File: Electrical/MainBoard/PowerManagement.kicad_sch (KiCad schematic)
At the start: 71 parts, among them Q1 AO3401A, U5 TPS65131RGE, U6 TPS2121RUXR, U7 TPS7A9401DSCR, U8 LM61460AASQRJRRQ1

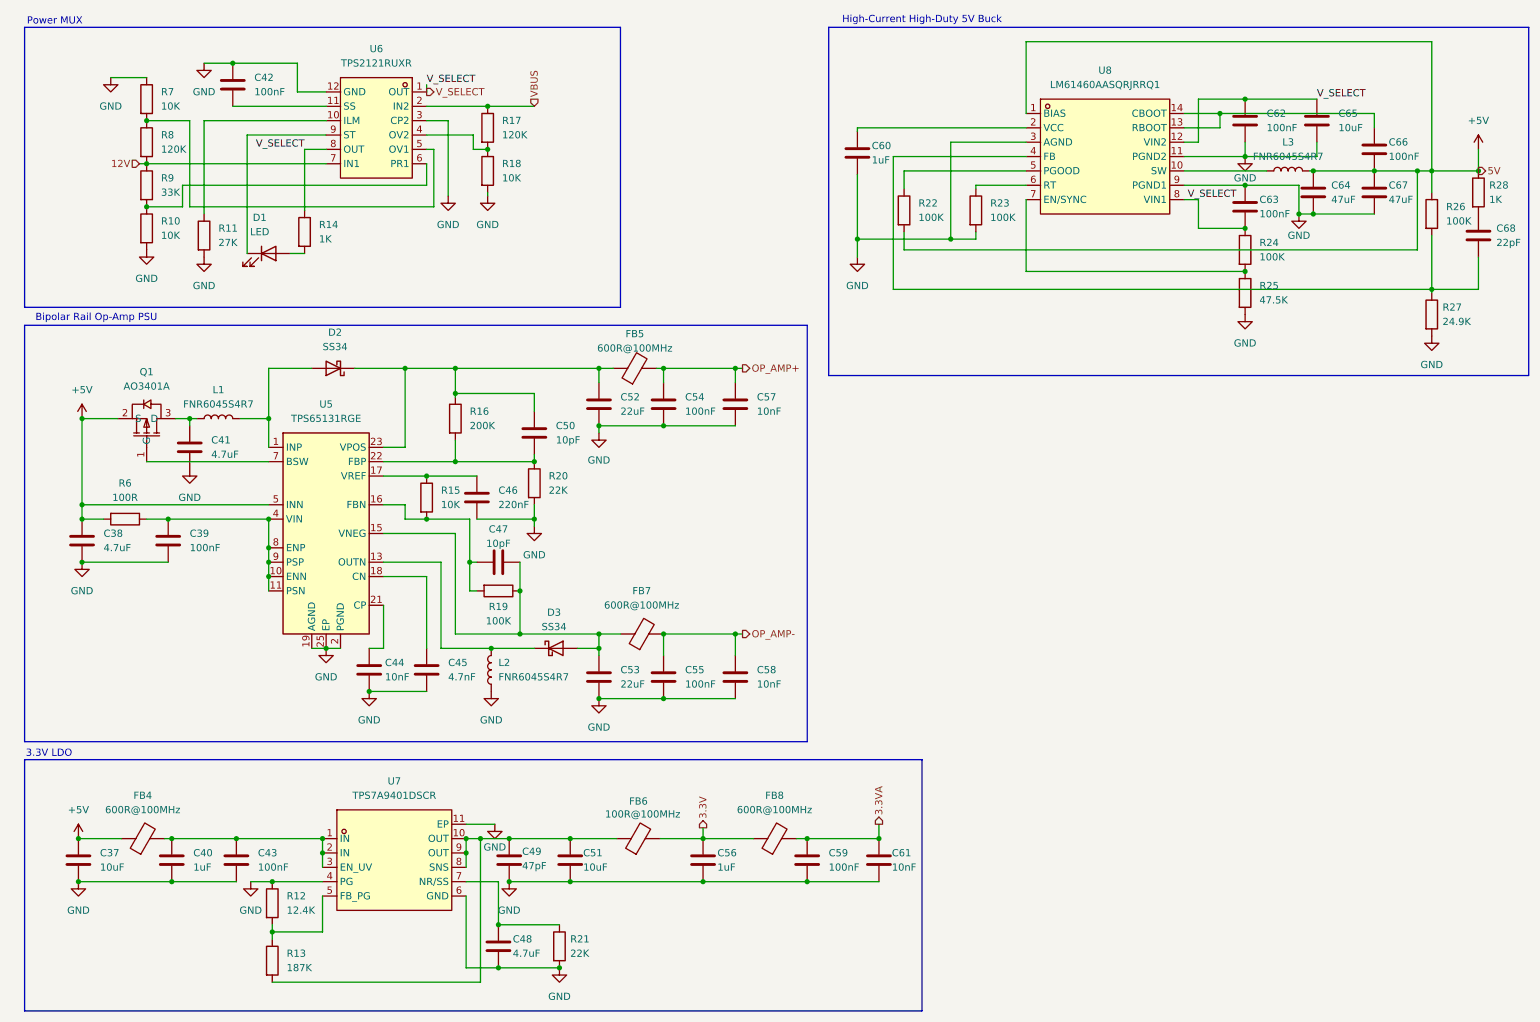
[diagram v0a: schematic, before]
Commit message: layout main
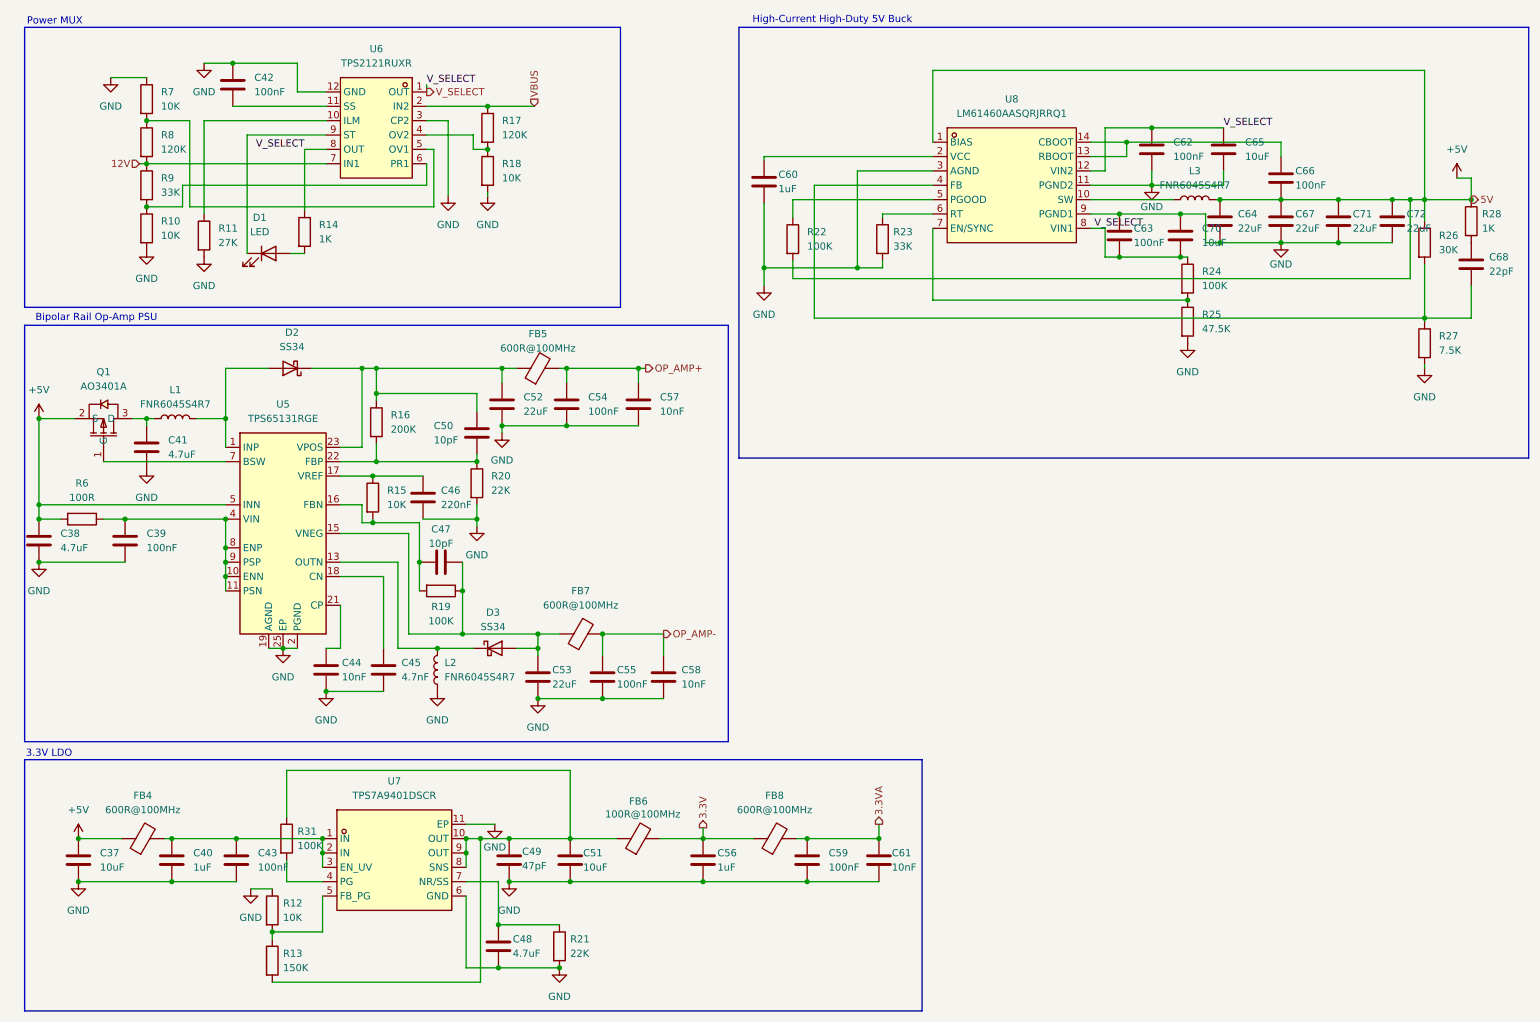
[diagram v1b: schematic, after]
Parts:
- added C70: 10uF, Capacitor_SMD:C_0603_1608Metric, symbol Device:C
- added C71, C72: 22uF, Capacitor_SMD:C_0805_2012Metric, symbol Device:C
- added R31: 100K, Resistor_SMD:R_0402_1005Metric, symbol Device:R
- C64, C67: value 47uF -> 22uF
- R10, R17, R18, R7, R8, R9: footprint Resistor_SMD:R_0402_1005Metric -> Resistor_SMD:R_0603_1608Metric
- R12: value 12.4K -> 10K; footprint Resistor_SMD:R_0603_1608Metric -> Resistor_SMD:R_0402_1005Metric
- R13: value 187K -> 150K
- R23: value 100K -> 33K
- R26: value 100K -> 30K; footprint Resistor_SMD:R_0402_1005Metric -> Resistor_SMD:R_0603_1608Metric
- R27: value 24.9K -> 7.5K
- R6: footprint Resistor_SMD:R_0603_1608Metric -> Resistor_SMD:R_0402_1005Metric
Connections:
- net +5V: now also C71.1, C72.1
- net GND: now also C70.1, C71.2, C72.2; no longer U7.4 (PG)
- net V_SELECT: now also C70.2
- net at C49.1, C51.1, FB6.1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: now also R31.1
- new net: R31.2, U7.4 (PG)
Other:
- moved on the sheet: C38, C39, C41, C44, C45, C46, C47, C50, C52, C53, C54, C55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

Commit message: new layout
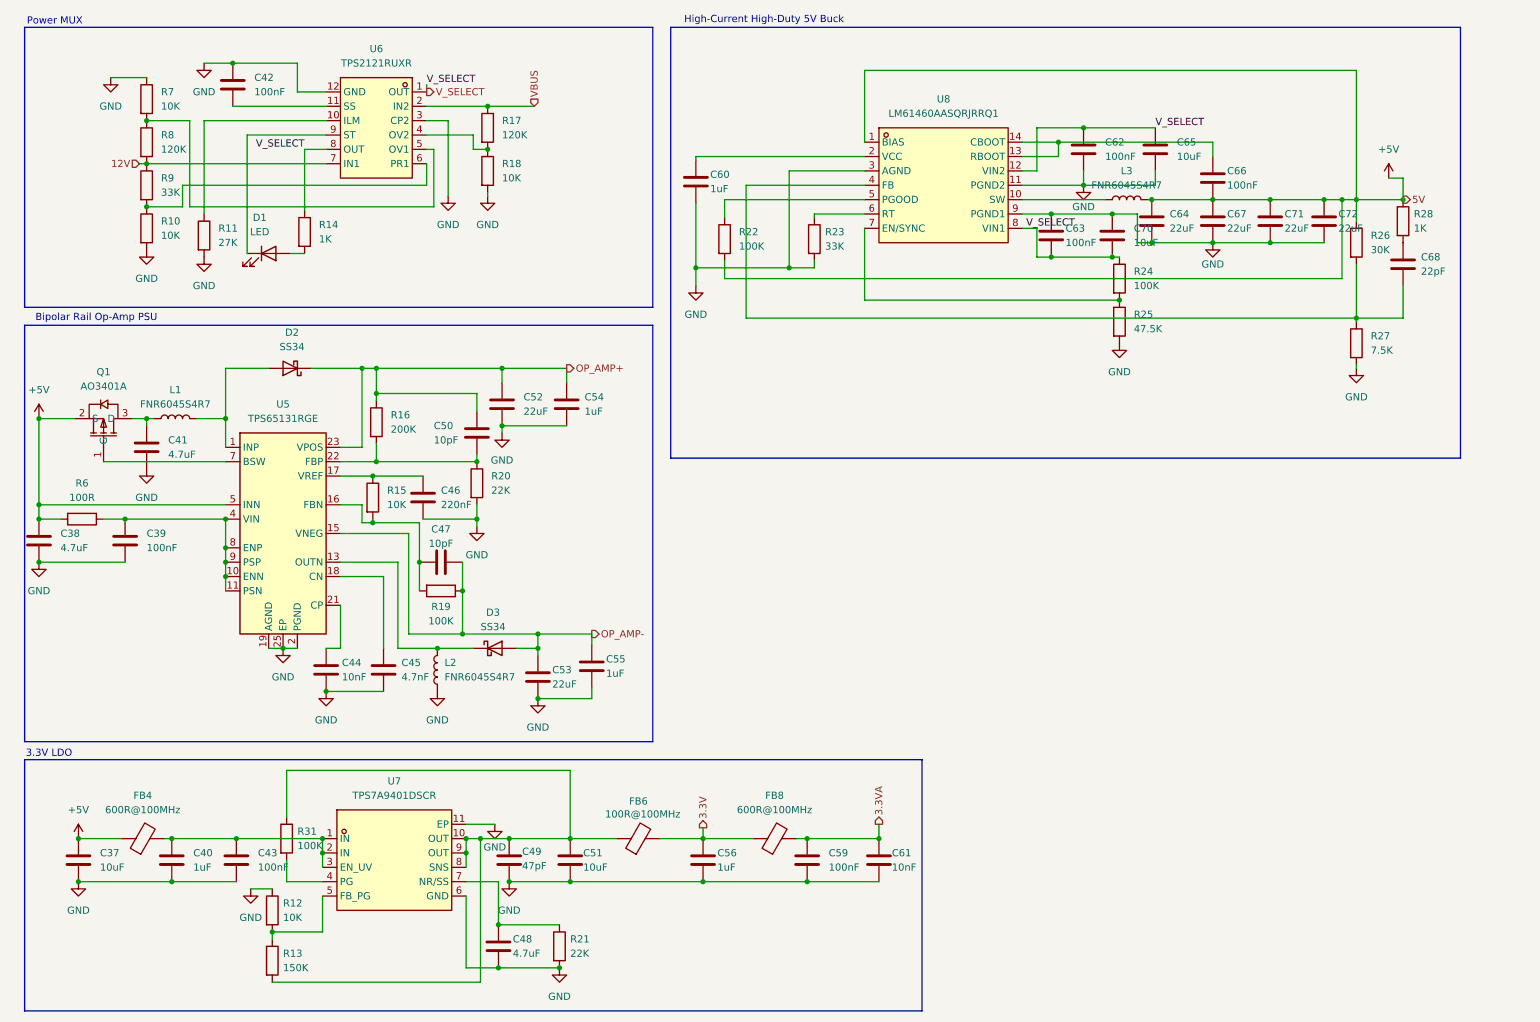
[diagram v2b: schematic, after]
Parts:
- removed C57, C58: 10nF, Capacitor_SMD:C_0402_1005Metric, symbol Device:C
- removed FB5, FB7: 600R@100MHz, Inductor_SMD:L_0805_2012Metric, symbol Device:FerriteBead
- C54, C55: value 100nF -> 1uF; footprint Capacitor_SMD:C_0402_1005Metric -> Capacitor_SMD:C_0603_1608Metric
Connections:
- net OP_AMP+: now also C50.1, C52.1, D2.1 (K), R16.1, U5.23 (VPOS)
- net OP_AMP-: now also C47.2, C53.1, D3.2 (A), R19.1, U5.15 (VNEG)
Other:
- moved on the sheet: C55, C60, C62, C63, C64, C65, C66, C67, C68, C70, C71, C72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
